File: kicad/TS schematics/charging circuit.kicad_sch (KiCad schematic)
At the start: 30 parts, among them J22 Activation Logic, J25 紅色儲能接綫柱100A, J26 AT04-3P-PM05, J27 Amphenol RT00122PM03, J28 紅色儲能接綫柱100A, K2 EV200-HAANA, K3 EV200-HAANA, K4 EV200-HAANA, K5 PNC113BDA, SW1 LVMS, SW10 TSMP Interlock, SW11 Motor Controller HVP800 Inter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, SW12 PL00X-301-50 Interlock, SW13 PL00Y-301-50 Interlock, SW14 PL00X-301-50 Interlock, SW15 PL00Y-301-50 Interlock, SW16 MINIMSDF000F HVD Interlock, SW17 BSPD, SW18 BAMOCAR, SW2 IMD, SW3 AMS, SW4 TSMS, SW5 Cockpit Shutdown Button, SW6 Left Shutdown Button, SW7 Right Shutdown Button, SW8 Inertia Switch, SW9 BOTS

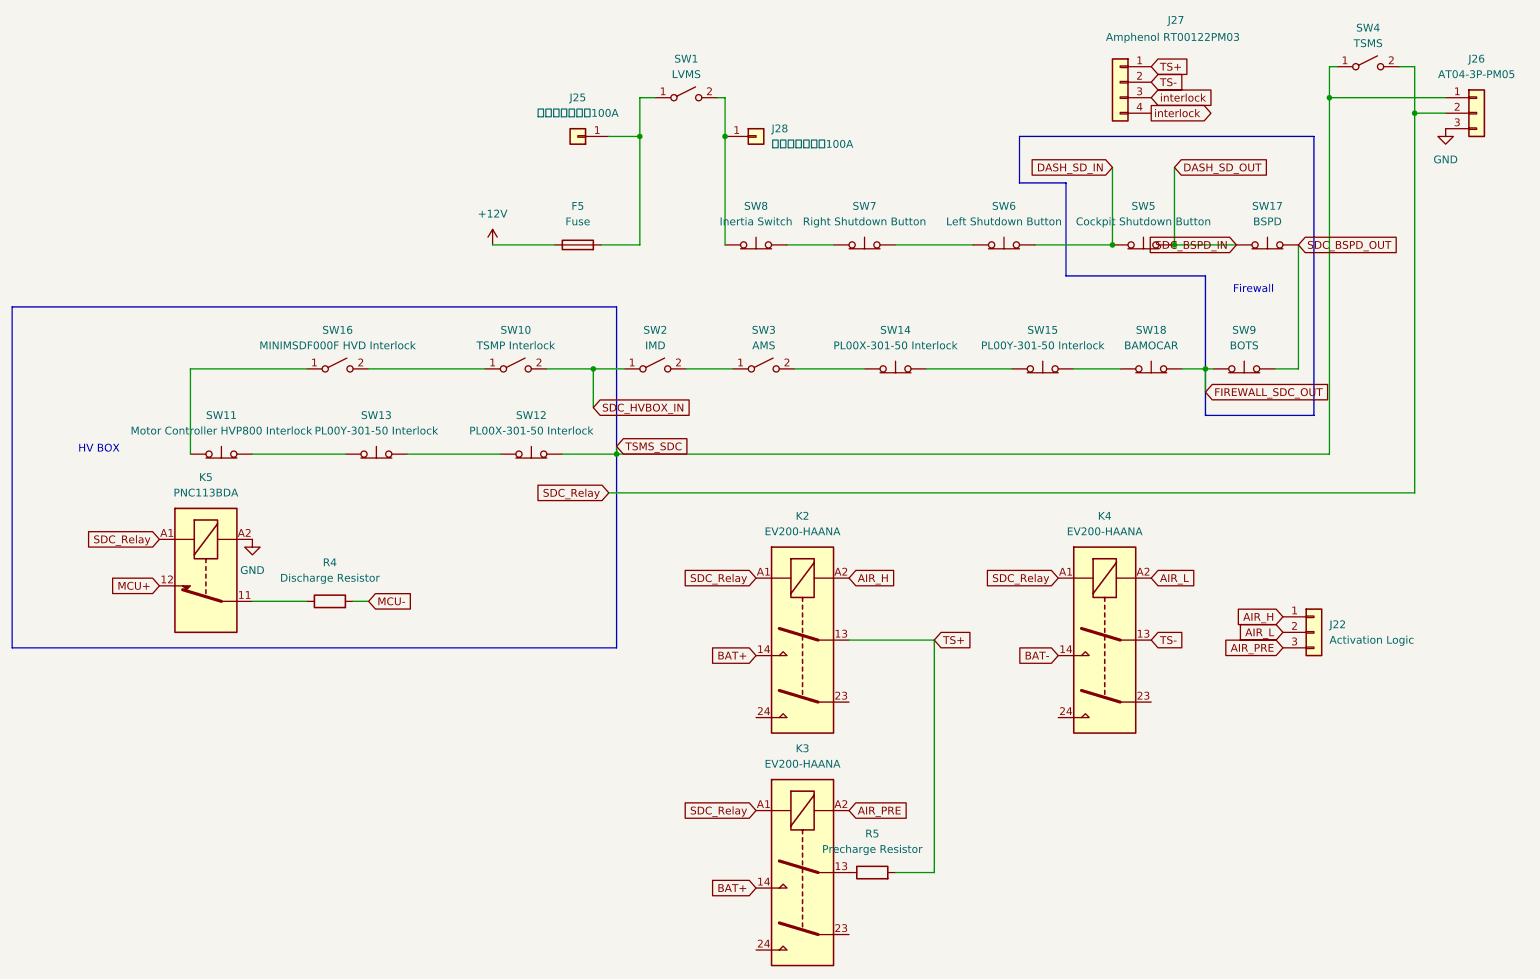
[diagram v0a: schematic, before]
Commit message: VCU V3.2 FINISH LAYOUT
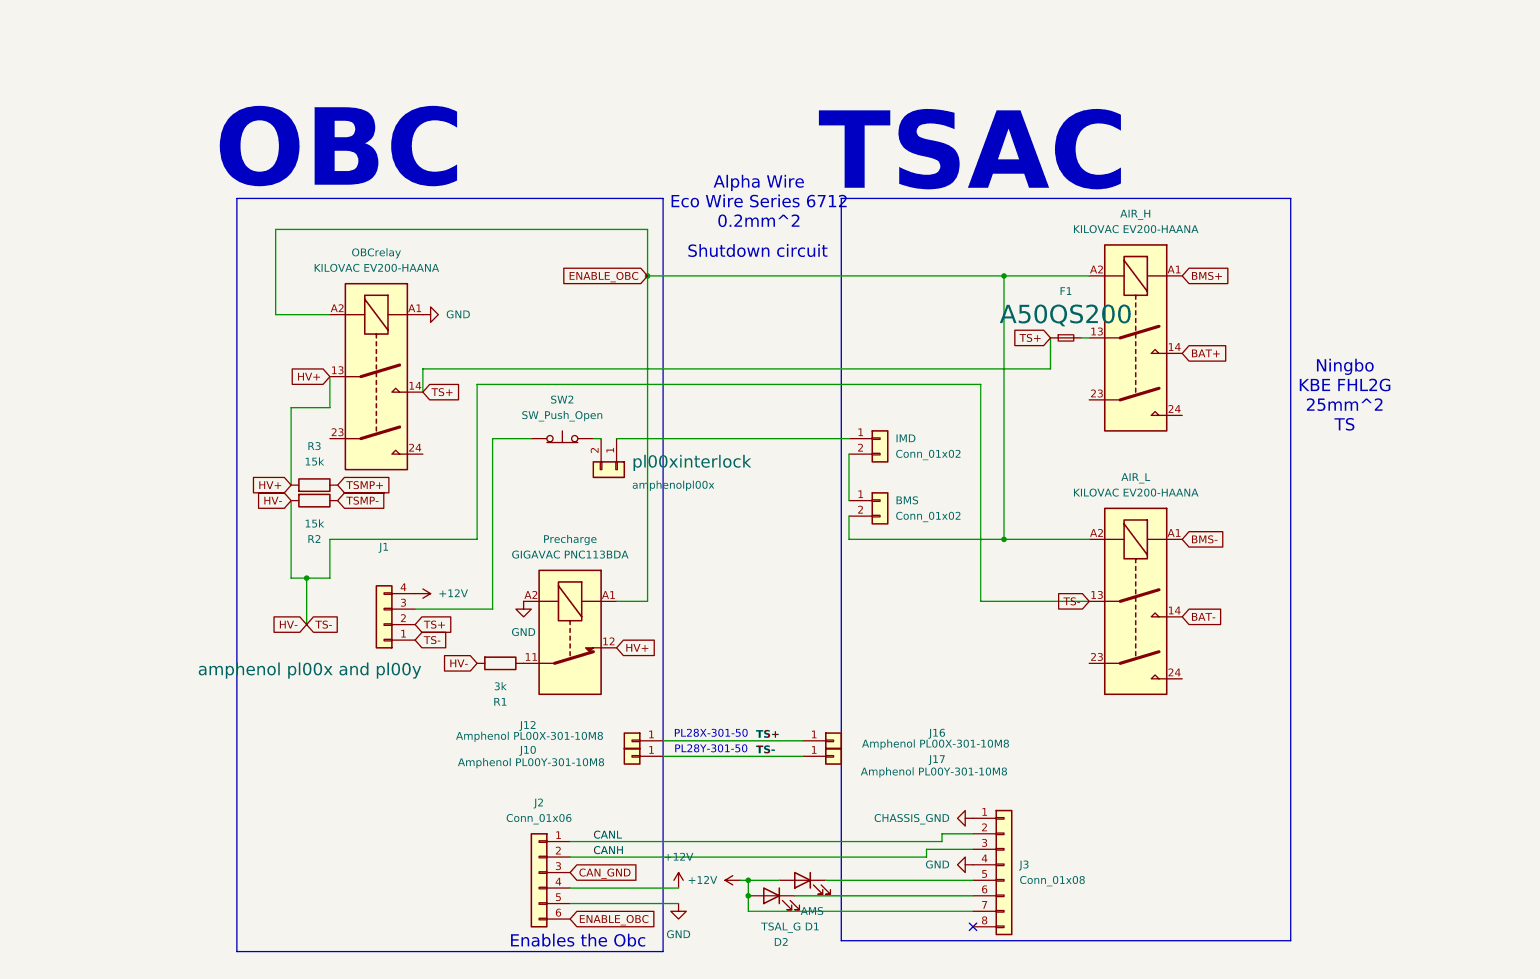
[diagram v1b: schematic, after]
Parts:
- removed F5: Fuse, symbol Device:Fuse
- removed J22: Activation Logic, symbol Connector_Generic:Conn_01x03
- removed J25, J28: 紅色儲能接綫柱100A, symbol Connector_Generic:Conn_01x01
- removed J26: AT04-3P-PM05, symbol Connector_Generic:Conn_01x03
- removed J27: Amphenol RT00122PM03, symbol Connector_Generic:Conn_01x04
- removed K2, K3, K4: EV200-HAANA, Relay_THT:Relay_DPST_Omron_G2RL-2A, symbol Relay:G2RL-2A
- removed K5: PNC113BDA, symbol Relay:Relay_SPST-NC
- removed R4: Discharge Resistor, symbol Device:R
- removed R5: Precharge Resistor, symbol Device:R
- removed SW1: LVMS, symbol Switch:SW_SPST
- removed SW10: TSMP Interlock, symbol Switch:SW_SPST
- removed SW11: Motor Controller HVP800 Interlock, symbol Switch:SW_Push_Open
- removed SW12, SW14: PL00X-301-50 Interlock, symbol Switch:SW_Push_Open
- removed SW13, SW15: PL00Y-301-50 Interlock, symbol Switch:SW_Push_Open
- removed SW16: MINIMSDF000F HVD Interlock, symbol Switch:SW_SPST
- removed SW17: BSPD, symbol Switch:SW_Push_Open
- removed SW18: BAMOCAR, symbol Switch:SW_Push_Open
- removed SW2: IMD, symbol Switch:SW_SPST
- removed SW3: AMS, symbol Switch:SW_SPST
- removed SW4: TSMS, symbol Switch:SW_SPST
- removed SW5: Cockpit Shutdown Button, symbol Switch:SW_Push_Open
- removed SW6: Left Shutdown Button, symbol Switch:SW_Push_Open
- removed SW7: Right Shutdown Button, symbol Switch:SW_Push_Open
- removed SW8: Inertia Switch, symbol Switch:SW_Push_Open
- removed SW9: BOTS, symbol Switch:SW_Push_Open
- added AIR_H, AIR_L, OBCrelay: KILOVAC EV200-HAANA, symbol Relay:Relay_DPST-NO
- added BMS, IMD: Conn_01x02, symbol Connector_Generic:Conn_01x02
- added D1: AMS, symbol Device:LED
- added D2: TSAL_G, symbol Device:LED
- added F1: A50QS200, symbol Device:Fuse_Small
- added J1: amphenol pl00x and pl00y, symbol Connector_Generic:Conn_01x04
- added J10, J17: Amphenol PL00Y-301-10M8, symbol Connector_Generic:Conn_01x01
- added J12, J16: Amphenol PL00X-301-10M8, symbol Connector_Generic:Conn_01x01
- added J2: Conn_01x06, symbol Connector_Generic:Conn_01x06
- added J3: Conn_01x08, symbol Connector_Generic:Conn_01x08
- added Precharge: GIGAVAC PNC113BDA, symbol Relay:Relay_SPST-NC
- added R1: 3k, symbol Device:R
- added R2, R3: 15k, symbol Device:R
- added SW2: SW_Push_Open, symbol Switch:SW_Push_Open
- added pl00xinterlock: amphenolpl00x, symbol Connector_Generic:Conn_01x02
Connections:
- net +12V: now also D1.2 (A), D2.2 (A), J1.4 (Pin_4), J2.4 (Pin_4), J3.7 (Pin_7)
- net BAT+: now also AIR_H.14
- net BAT-: now also AIR_L.14
- net GND: now also J2.5 (Pin_5), J3.4 (Pin_4), OBCrelay.A1, Precharge.A2
- net TS+: now also F1.1, J1.2 (Pin_2), J12.1 (Pin_1), J16.1 (Pin_1), OBCrelay.14
- new net: D1.1 (K), J3.5 (Pin_5)
- new net: IMD.1 (Pin_1), pl00xinterlock.1 (Pin_1)
- new net: BMS.1 (Pin_1), IMD.2 (Pin_2)
- new net: D2.1 (K), J3.6 (Pin_6)
- new net: AIR_H.13, F1.2
- new net: Precharge.11, R1.1
- new net: J1.3 (Pin_3), SW2.1 (A)
- new net: SW2.2 (B), pl00xinterlock.2 (Pin_2)
- new net BMS+: AIR_H.A1
- new net BMS-: AIR_L.A1
- new net CANH: J2.2 (Pin_2), J3.3 (Pin_3)
- new net CANL: J2.1 (Pin_1), J3.2 (Pin_2)
- new net CAN_GND: J2.3 (Pin_3)
- new net CHASSIS_GND: J3.1 (Pin_1)
- new net ENABLE_OBC: AIR_H.A2, AIR_L.A2, BMS.2 (Pin_2), J2.6 (Pin_6), OBCrelay.A2, Precharge.A1
- new net HV+: OBCrelay.13, Precharge.12, R3.2
- new net HV-: AIR_L.13, J1.1 (Pin_1), J10.1 (Pin_1), J17.1 (Pin_1), R1.2, R2.2
- new net TSMP+: R3.1
- new net TSMP-: R2.1
- no-connect marks 0 -> 1
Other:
- note added: "Alpha Wire Eco Wire Series 6712 0.2mm^2"
- note added: "Enables the Obc"
- note added: "Ningbo KBE FHL2G 25mm^2 TS"
- note added: "OBC"
- note added: "PL28X-301-50"
- note added: "PL28Y-301-50"
- note added: "Shutdown circuit"
- note added: "TSAC"
- note removed: "Firewall"
- note removed: "HV BOX"
